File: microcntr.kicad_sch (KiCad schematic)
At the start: 165 parts, among them IC1 M24512-RDW6TP, IC2 ADF4156BRUZ, IC3 ADM7160AUJZ-3.3-R7, IC4 ADM7160AUJZ-3.3-R7, J1 U.FL, J10 U.FL, J4 Conn_01x16, J5 RF2-04A-T-00-50-G, J6 Conn_01x12, J7 USB_B_Micro, J8 RF2-04A-T-00-50-G, J9 RF2-04A-T-00-50-G, Q1 BSH105,215, Q2 BC69PASX, Q3 BCV62C, Q4 BFU550WF, U1 SN74LVC1G80QDCKRQ1, U11 SN74LVC1G97DCKR, U12 TLV3601DCKR, U14 MAX-M10S-00B, U15 TLV3601DCKR, U16 LMT85DCKR, U17 TLV9162IDDFR, U18 SN74LVC1G80QDCKRQ1, U2 ADR381ARTZ-R2, U3 TLV3601DCKR, U4 TLV9162IDDFR, U5 SN74LVC1G80QDCKRQ1, U6 SN74LVC1G97DCKR, U7 STM32F410RBT6, U8 SN74LVC1G97DCKR, U9 FT230XS, Y2 CCHD-575-50-100.000

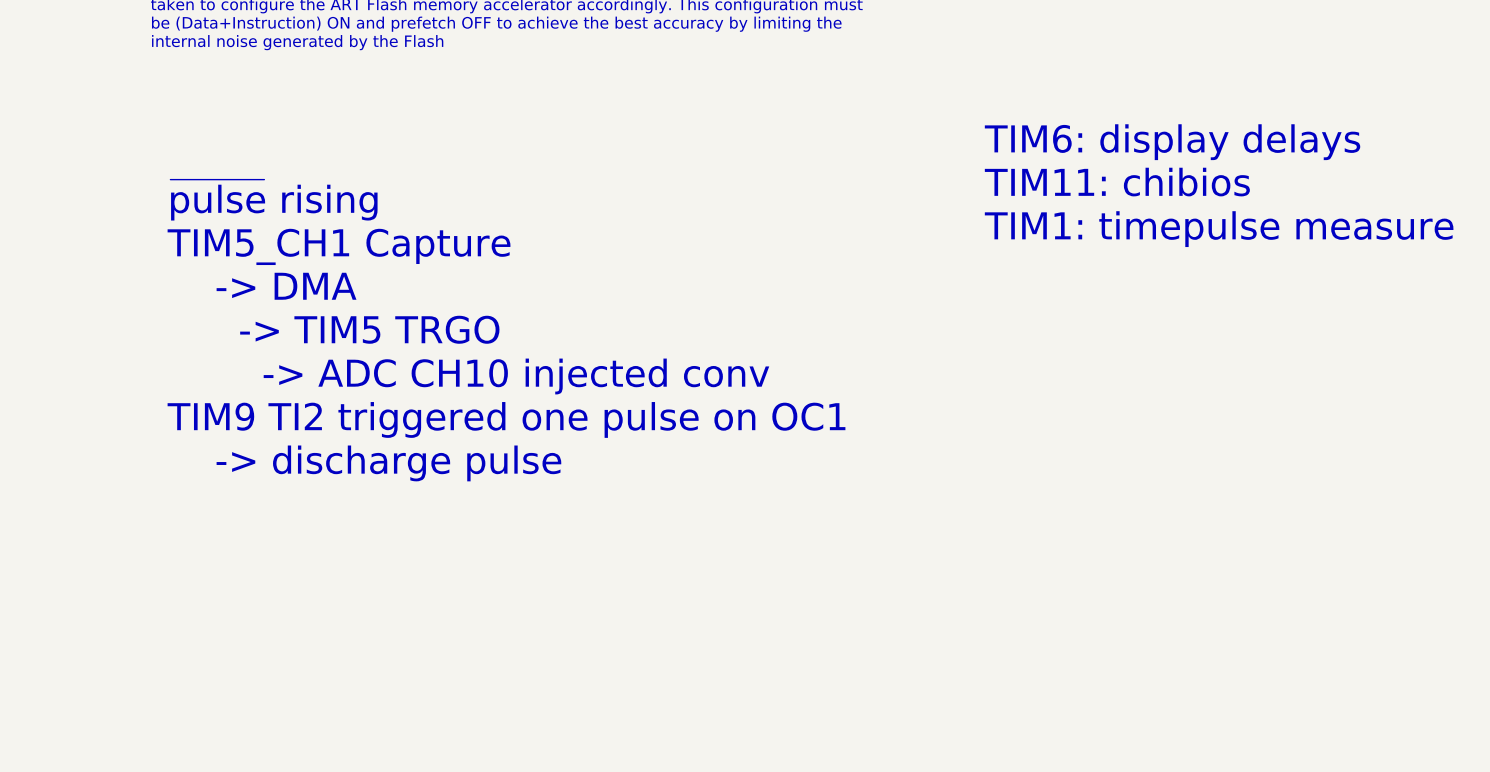
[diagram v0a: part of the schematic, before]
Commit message: filled in buglist
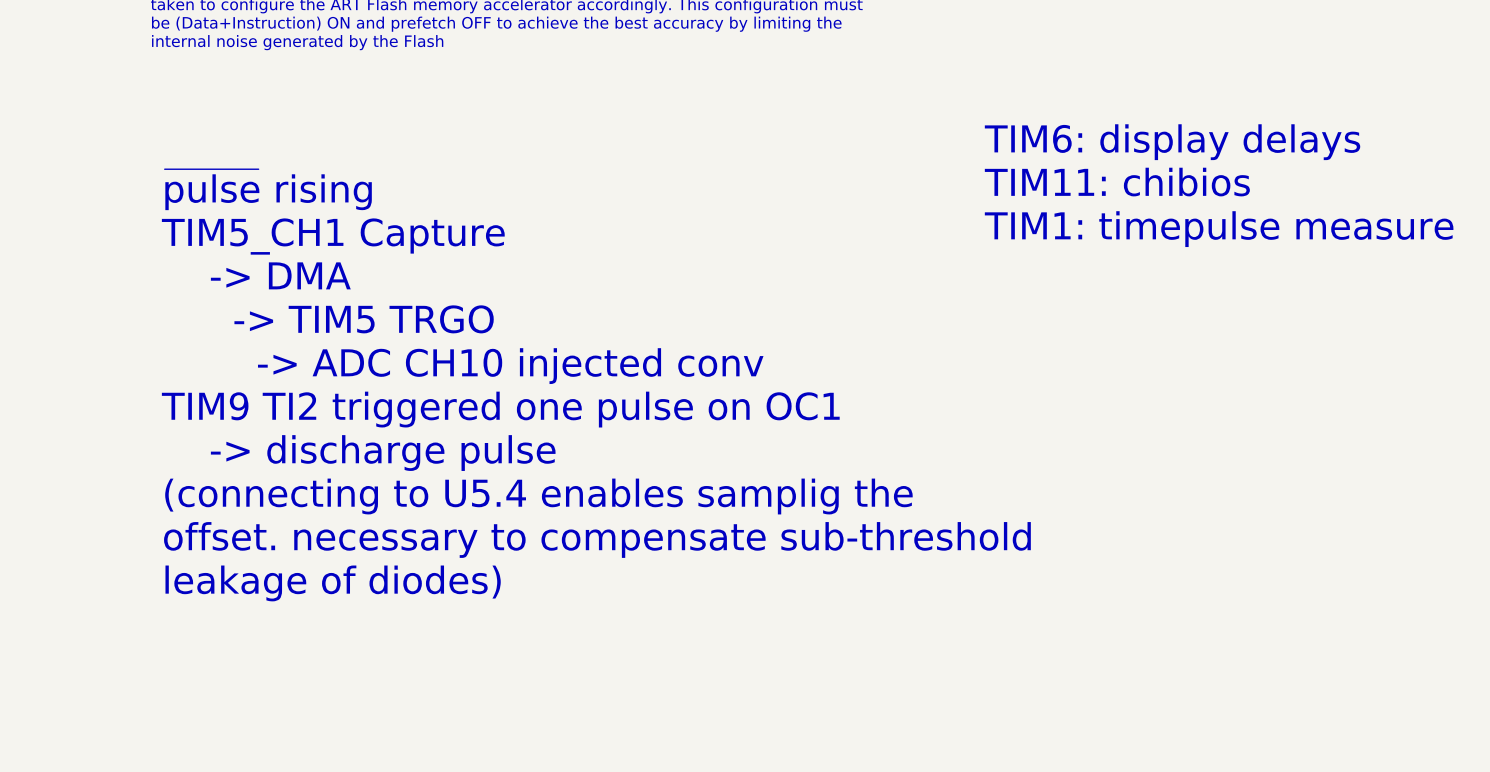
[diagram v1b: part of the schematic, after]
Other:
- note added: "~{pulse} rising TIM5_CH1 Capture -> DMA -> TIM5 TRGO -> ADC CH10 injected conv TIM9 TI2 triggered one pulse on OC1 -> discharge pulse (connecting to U5.4 enables samplig the offset. necessary to compensate sub-threshold leakage of diodes)"
- note removed: "~{pulse} rising TIM5_CH1 Capture -> DMA -> TIM5 TRGO -> ADC CH10 injected conv TIM9 TI2 triggered one pulse on OC1 -> discharge pulse"
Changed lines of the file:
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@@
     (effects (font (size 1.27 1.27) (thickness 0.254) bold) (justify left bottom))
   )
-  (text "~{pulse} rising\nTIM5_CH1 Capture \n	-> DMA\n  	-> TIM5 TRGO\n		-> ADC CH10 injected conv\nTIM9 TI2 triggered one pulse on OC1\n	-> discharge pulse"
-    (at 187.96 135.255 0)
+  (text "~{pulse} rising\nTIM5_CH1 Capture \n	-> DMA\n  	-> TIM5 TRGO\n		-> ADC CH10 injected conv\nTIM9 TI2 triggered one pulse on OC1\n	-> discharge pulse\n(connecting to U5.4 enables samplig the \noffset. necessary to compensate sub-threshold\nleakage of diodes)"
+    (at 187.325 148.59 0)
     (effects (font (size 3 3)) (justify left bottom))
   )
